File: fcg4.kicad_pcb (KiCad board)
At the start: 4 copper layers, 34 x 34 mm, 107 parts, among them IC1 MP9943AGQ-Z, IC2 MP9943AGQ-Z, J1 USB4105-GF-A-120, J2 SM08B-SRSS-TB, U1 STM32G473CEUx, U10 MAX40200ANS_T, U11 MAX40200ANS_T, U2 ICM-42688-P, U23 SDA, U26 SCL, U31 9V, U4 AP2112K-3.3TRG1, U5 AP2112K-1.8TRG1, Y1 ECS-240-6-37B-7KM-TR

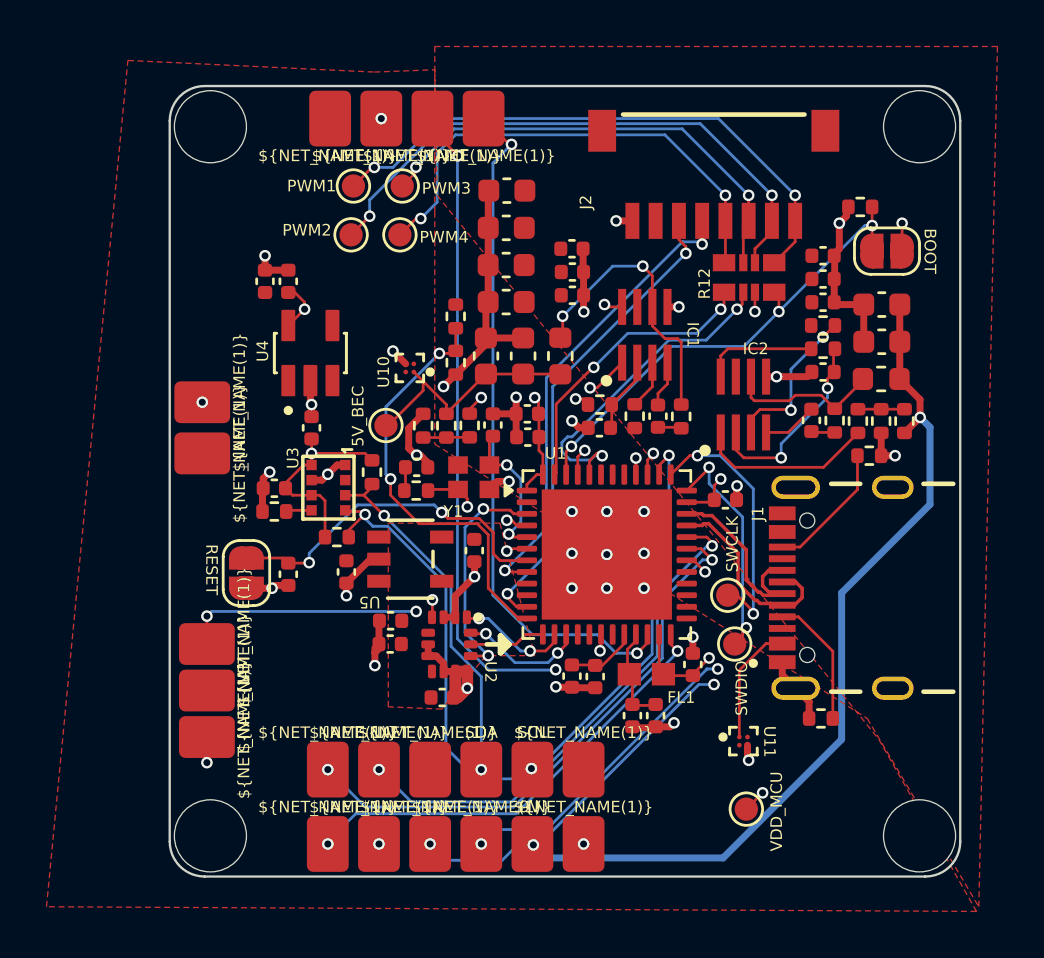
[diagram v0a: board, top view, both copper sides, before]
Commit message: routing...
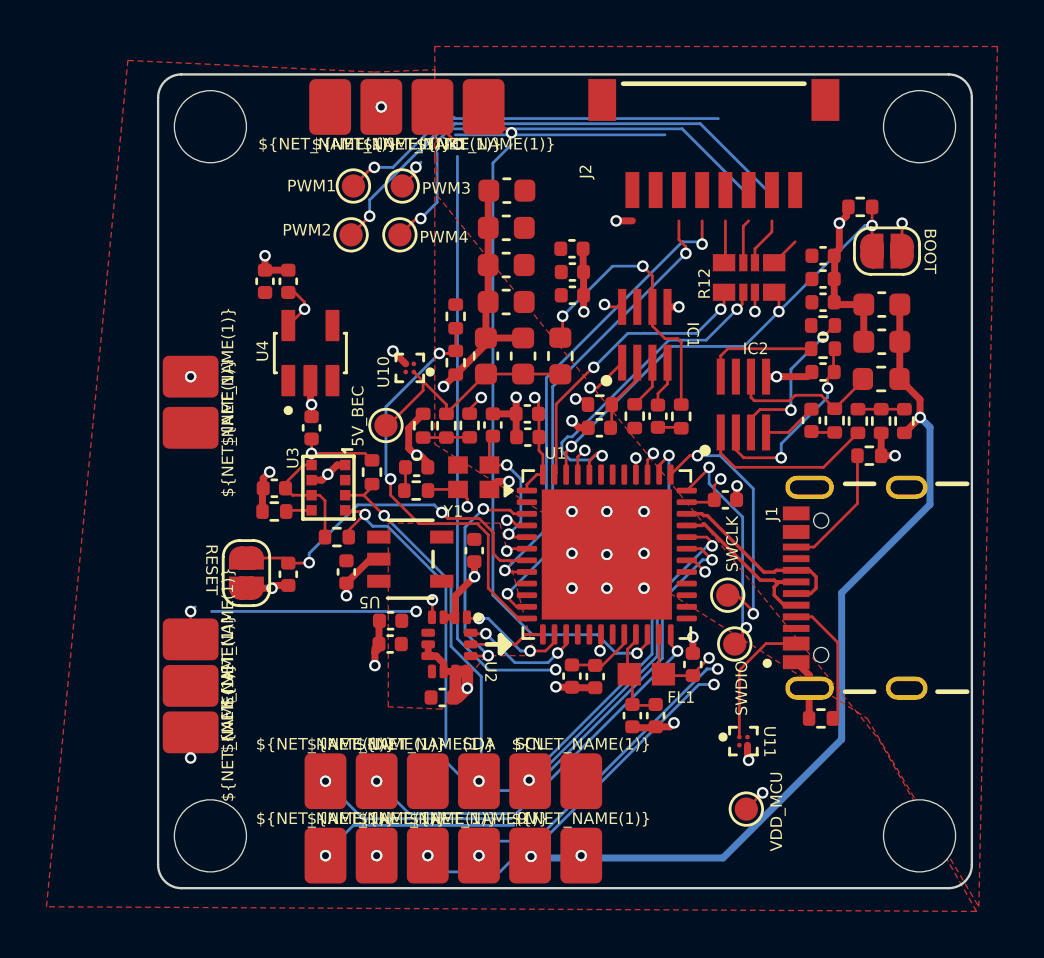
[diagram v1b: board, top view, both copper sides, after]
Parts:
- moved J2 1.32 mm to (23.4, -0.30)
- moved U18 1.21 mm to (0.90, 14.7)
- moved U19 1.21 mm to (0.90, 12.5)
- moved U22 0.73 mm to (0.90, 23.8)
- moved U24 0.73 mm to (0.90, 25.8)
- moved U25 0.73 mm to (0.90, 27.8)
- moved J1 0.60 mm to (31.7, 21.6)
- moved U28 0.51 mm to (17.7, 33.1)
- moved U9 0.51 mm to (17.7, 29.9)
- moved U23 0.51 mm to (13.3, 29.9)
- moved U26 0.51 mm to (15.5, 29.9)
- moved U27 0.51 mm to (6.70, 33.1)
- moved U29 0.51 mm to (11.1, 33.1)
- moved U30 0.51 mm to (13.3, 33.1)
- moved U31 0.51 mm to (15.5, 33.1)
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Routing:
- net TX3: track 29.6 -> 52.5 mm
- net /Connectors/MOTOR_3: track 20.2 -> 5.28 mm, vias 2 -> 1
- net /Connectors/MOTOR_4: track 21.0 -> 7.23 mm, vias 2 -> 1
- net /Connectors/MOTOR_1: track 24.8 -> 18.2 mm, vias 2 -> 1
- net /Connectors/MOTOR_2: track 25.0 -> 23.9 mm, vias 2 -> 1
- net 5V_USB: track 5.19 -> 5.79 mm
- net /MCU/USB_DIFF+: track 8.69 -> 8.19 mm
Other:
- board size 34 x 34 mm -> 35 x 35 mm
